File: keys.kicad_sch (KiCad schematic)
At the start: 0 parts

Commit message: [ADD](General) v1
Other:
- company: (none) -> Ryzzen
- title: (none) -> TMR based triple USB Keyboard
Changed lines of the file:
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@@
 	(generator_version "9.0")
 	(paper "A4")
+	(title_block
+		(title "TMR based triple USB Keyboard")
+		(date "2025-12-28")
+		(rev "v1")
+		(company "Ryzzen")
+	)
 	(junction
 		(at 194.31 82.55)
@@
 			(project "RyzzenKeyboard"
 				(path "/5d44d704-6136-40a8-98a4-93f001ea8743/c5dd3d76-8c7d-4253-bbc0-6b560edbfa92"
-					(page "4")
+					(page "108")
 				)
 			)
@@
 			(project "RyzzenKeyboard"
 				(path "/5d44d704-6136-40a8-98a4-93f001ea8743/c5dd3d76-8c7d-4253-bbc0-6b560edbfa92"
-					(page "2")
-				)
-			)
+					(page "4")
+				)
+			)

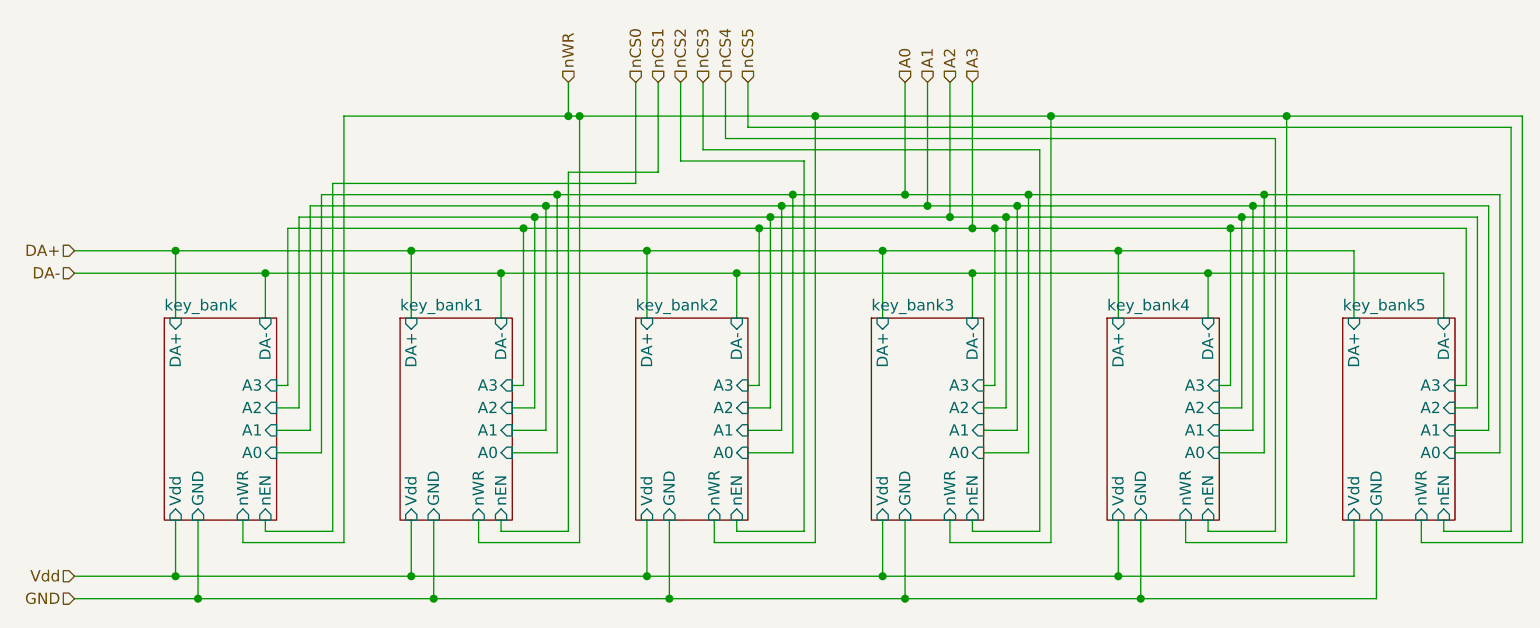
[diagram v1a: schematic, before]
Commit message: [ADD](General) v2 split
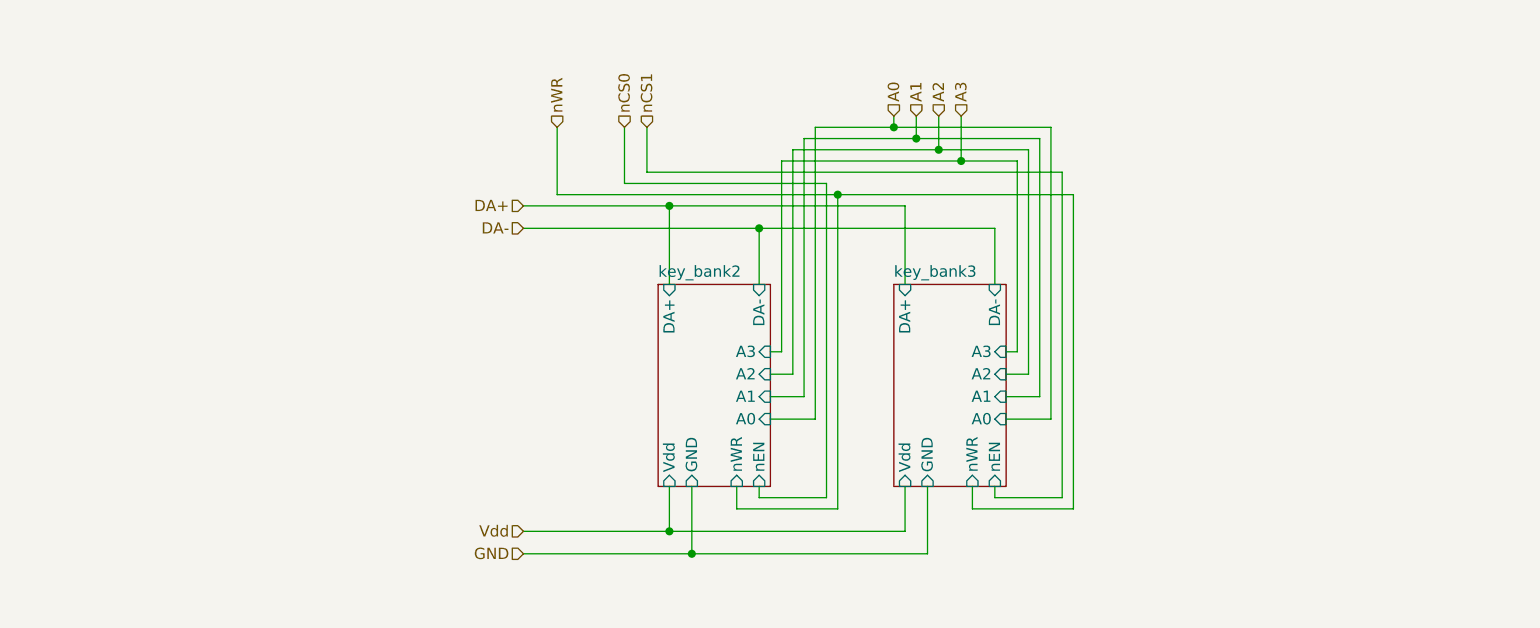
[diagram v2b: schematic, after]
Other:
- removed sheet key_bank
- removed sheet key_bank1
- removed sheet key_bank4
- removed sheet key_bank5
